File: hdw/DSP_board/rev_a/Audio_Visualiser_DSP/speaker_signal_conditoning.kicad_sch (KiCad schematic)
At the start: 6 parts, among them J1401 Left, T1401 Transformer_Audio

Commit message: assigned some footprints
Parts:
- R1401, R1402: footprint (none) -> Resistors_SMD:R_0805
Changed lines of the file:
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@@
 			)
 		)
-		(property "Footprint" ""
+		(property "Footprint" "Resistors_SMD:R_0805"
 			(at 132.08 63.5 0)
 			(hide yes)
@@
 				(font
 					(size 1.524 1.524)
+				)
+			)
+		)
+		(property "Sim.Type" ""
+			(at 132.08 63.5 90)
+			(hide yes)
+			(show_name no)
+			(do_not_autoplace no)
+			(effects
+				(font
+					(size 1.27 1.27)
 				)
 			)
@@
 			)
 		)
+		(property "Sim.Type" ""
+			(at 119.38 63.5 90)
+			(hide yes)
+			(show_name no)
+			(do_not_autoplace no)
+			(effects
+				(font
+					(size 1.27 1.27)
+				)
+			)
+		)
 		(pin "2"
 		)
@@
 			)
 		)
+		(property "Sim.Type" ""
+			(at 179.07 63.5 90)
+			(hide yes)
+			(show_name no)
+			(do_not_autoplace no)
+			(effects
+				(font
+					(size 1.27 1.27)
+				)
+			)
+		)
 		(pin "2"
 		)
@@
 			)
 		)
-		(property "Footprint" ""
+		(property "Footprint" "Resistors_SMD:R_0805"
 			(at 140.97 57.15 0)
 			(hide yes)
@@
 		)
 		(property "Digi-Key PN" ""
+			(at 140.97 57.15 0)
+			(hide yes)
+			(show_name no)
+			(do_not_autoplace no)
+			(effects
+				(font
+					(size 1.27 1.27)
+				)
+			)
+		)
+		(property "Sim.Type" ""
 			(at 140.97 57.15 0)
 			(hide yes)
@@
 		)
 		(property "Description" "Audio transformer"
+			(at 87.63 68.58 0)
+			(hide yes)
+			(show_name no)
+			(do_not_autoplace no)
+			(effects
+				(font
+					(size 1.27 1.27)
+				)
+			)
+		)
+		(property "Sim.Type" ""
 			(at 87.63 68.58 0)
 			(hide yes)
@@
 			(at 59.69 67.31 0)
 			(hide yes)
+			(show_name no)
+			(do_not_autoplace no)
+			(effects
+				(font
+					(size 1.27 1.27)
+				)
+			)
+		)
+		(property "Sim.Type" ""
+			(at 59.69 67.31 0)
+			(hide yes)

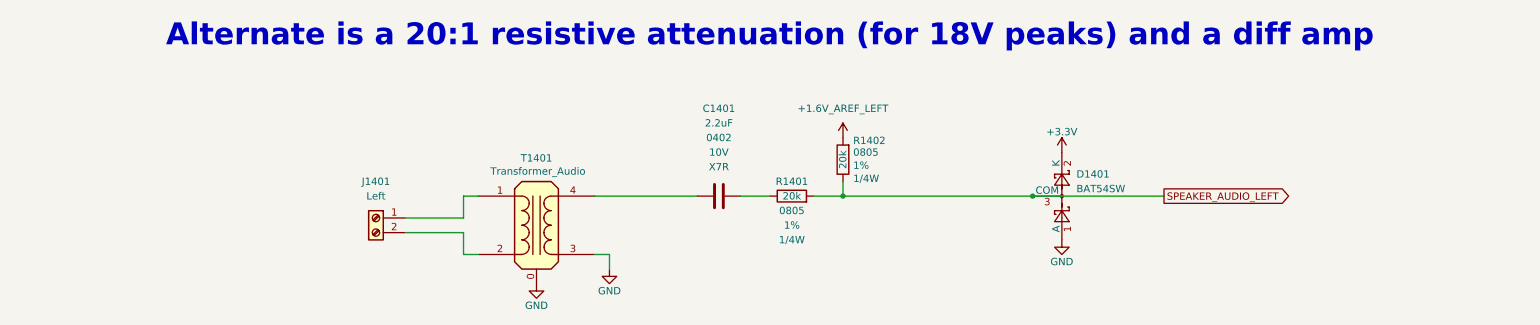
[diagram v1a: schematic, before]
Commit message: assigned many digi-key part numbers
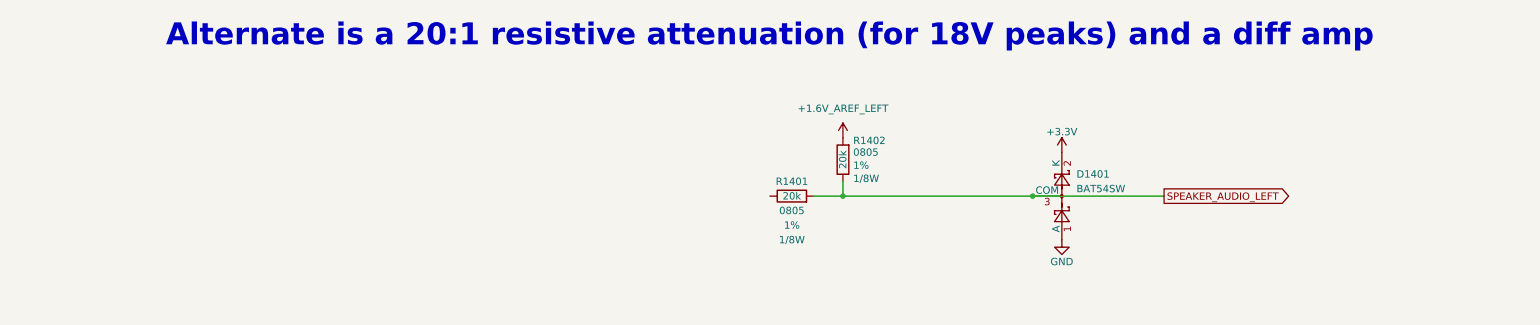
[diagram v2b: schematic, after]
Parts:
- removed C1401: 2.2uF, Capacitors_SMD:C_0402, symbol Custom Library:C_Custom
- removed J1401: Left, symbol Connector:Screw_Terminal_01x02
- removed T1401: Transformer_Audio, symbol Device:Transformer_Audio
- D1401: Digi-Key PN (none) -> BAT54SWT1GOSCT-ND
- R1401, R1402: Digi-Key PN (none) -> 311-20.0KCRCT-ND; Wattage 1/4W -> 1/8W
